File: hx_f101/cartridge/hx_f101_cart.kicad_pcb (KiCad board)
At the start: 2 copper layers, 100 x 85 mm, 10 parts, among them J1 Conn_02x25_Odd_Even, J2 CONN_02x17, U1 27C128, U2 74LS245, U3 74LS133, U4 74LS32, U5 74LS04, U6 74LS07, U7 74LS07, U8 74LS00

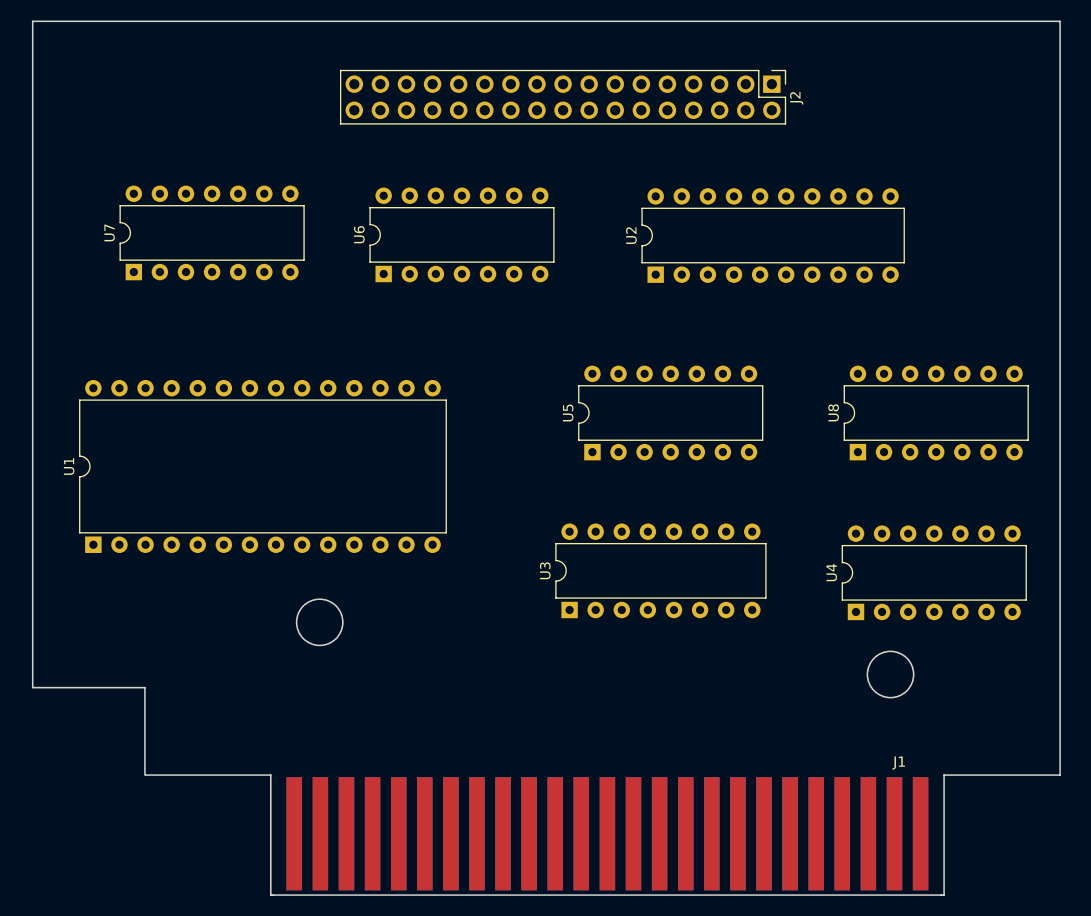
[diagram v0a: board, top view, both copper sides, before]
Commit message: Add files via upload
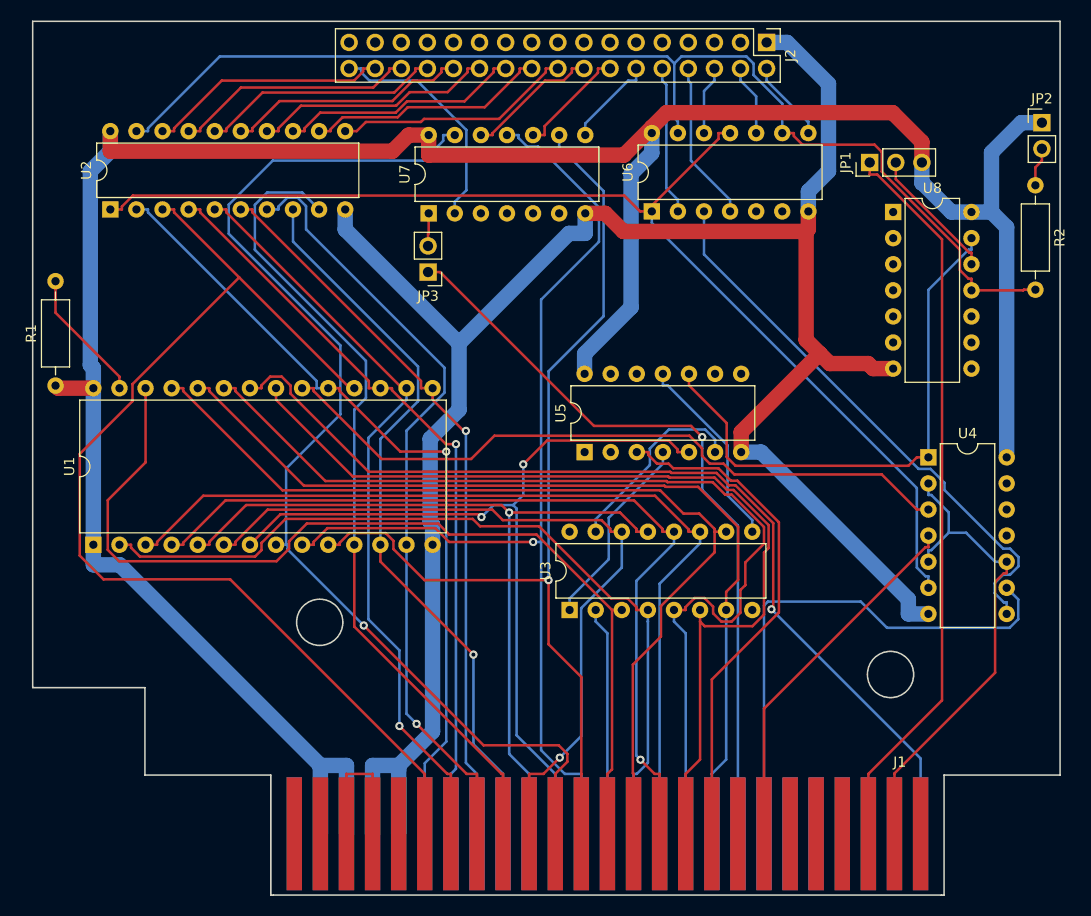
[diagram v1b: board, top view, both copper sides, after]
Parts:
- added JP1: Jumper_NC_Dual, Connector_PinHeader_2.54mm:PinHeader_1x03_P2.54mm_Vertical, F.Cu at (200.5, 70.7)
- added JP2: Jumper, Connector_PinHeader_2.54mm:PinHeader_1x02_P2.54mm_Vertical, F.Cu at (217.2, 66.9)
- added JP3: Jumper, Connector_PinHeader_2.54mm:PinHeader_1x02_P2.54mm_Vertical, F.Cu at (157.5, 81.4)
- added R1: 10K, Resistor_THT:R_Axial_DIN0207_L6.3mm_D2.5mm_P10.16mm_Horizontal, F.Cu at (121.2, 92.5)
- added R2: 330R, Resistor_THT:R_Axial_DIN0207_L6.3mm_D2.5mm_P10.16mm_Horizontal, F.Cu at (216.6, 73.0)
- moved U2 53.5 mm to (126.6, 75.3)
- moved U7 29.3 mm to (157.5, 75.7)
- moved U6 26.8 mm to (179.3, 75.5)
- moved U8 23.6 mm to (202.8, 75.6), turned to 0 degrees
- moved U4 16.6 mm to (206.2, 99.4), turned to 0 degrees
- moved J2 4.10 mm to (190.4, 59.1)
- moved U5 0.76 mm to (172.7, 98.9)
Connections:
- net P18 renamed PB18
- net P20 renamed PB20
- net P22 renamed PB22
- net P24 renamed PB24
- net P26 renamed PB26
- net P28 renamed PB28
- net P30 renamed PB30
- net P32 renamed PB32
- J1 pad 13: (no net) -> _WR
- J1 pad 14: (no net) -> _RD
- J1 pad 15: (no net) -> _RESET
- J1 pad 18: (no net) -> A15
- J1 pad 25: (no net) -> A14
- J1 pad 6: (no net) -> _RFSH
- J2 pad 1: (no net) -> GND
- J2 pad 10: (no net) -> PB10
- J2 pad 12: (no net) -> PB12
- J2 pad 14: (no net) -> PB14
- J2 pad 16: (no net) -> PB16
- J2 pad 2: (no net) -> PB2
- J2 pad 34: (no net) -> PB34
- J2 pad 4: (no net) -> PB4
- J2 pad 6: (no net) -> PB6
- J2 pad 8: (no net) -> PB8
- U1 pad 20: _SLTSL -> _ROM_CE
- U1 pad 27: (no net) -> Net-(R1-Pad2)
- U2 pad 1: (no net) -> _RE
- U2 pad 19: Net-(U2-Pad19) -> _CS
- U3 pad 1: (no net) -> Net-(U3-Pad1)
- U3 pad 10: (no net) -> A8
- U3 pad 11: (no net) -> A7
- U3 pad 12: (no net) -> A6
- U3 pad 13: (no net) -> A5
- U3 pad 14: (no net) -> A4
- U3 pad 15: (no net) -> Net-(U3-Pad15)
- U3 pad 2: (no net) -> A14
- U3 pad 3: (no net) -> A13
- U3 pad 4: (no net) -> A12
- U3 pad 5: (no net) -> A11
- U3 pad 6: (no net) -> A10
- U3 pad 7: (no net) -> A9
- U3 pad 9: Net-(U2-Pad19) -> Net-(U3-Pad9)
- U4 pad 1: (no net) -> Net-(U4-Pad1)
- U4 pad 10: (no net) -> _SLTSL
- U4 pad 13: Net-(U2-Pad19) -> (no net)
- U4 pad 2: (no net) -> _SLTSL
- U4 pad 3: (no net) -> _ROM_CE
- U4 pad 4: (no net) -> _RD
- U4 pad 5: (no net) -> _SLTSL
- U4 pad 6: (no net) -> _RE
- U4 pad 8: Net-(U4-Pad8) -> _WE
- U4 pad 9: (no net) -> _WR
- U5 pad 10: Net-(U5-Pad10) -> Net-(U4-Pad1)
- U5 pad 11: (no net) -> Net-(U3-Pad9)
- U5 pad 3: (no net) -> A15
- U5 pad 4: (no net) -> Net-(U3-Pad1)
- U5 pad 5: (no net) -> A3
- U5 pad 6: (no net) -> Net-(U3-Pad15)
- U6 pad 1: (no net) -> _RE
- U6 pad 10: (no net) -> PB4
- U6 pad 11: (no net) -> _RE
- U6 pad 12: (no net) -> PB6
- U6 pad 13: (no net) -> _CS
- U6 pad 2: (no net) -> PB10
- U6 pad 3: (no net) -> _WE
- U6 pad 4: (no net) -> PB8
- U6 pad 8: (no net) -> PB2
- U6 pad 9: (no net) -> _CS
- U7 pad 1: (no net) -> Net-(JP3-Pad2)
- U7 pad 10: (no net) -> PB14
- U7 pad 11: (no net) -> A1
- U7 pad 12: (no net) -> PB16
- U7 pad 13: (no net) -> A2
- U7 pad 2: (no net) -> PB34
- U7 pad 8: (no net) -> PB12
- U7 pad 9: (no net) -> A0
- U8 pad 1: Net-(U4-Pad8) -> (no net)
- U8 pad 11: (no net) -> _CS
- U8 pad 12: (no net) -> Net-(JP1-Pad2)
- U8 pad 13: (no net) -> Net-(U4-Pad1)
- U8 pad 9: Net-(U5-Pad10) -> (no net)
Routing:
- net 5V: track 0.00 -> 254.4 mm
- net GND: track 0.00 -> 199.6 mm
- net _RE: track 0.00 -> 113.7 mm
- net _CS: track 0.00 -> 113.1 mm
- net A2: track 0.00 -> 110.2 mm, vias 0 -> 1
- net D6: track 0.00 -> 107.8 mm
- net A1: track 0.00 -> 102.6 mm, vias 0 -> 1
- net A11: track 0.00 -> 98.7 mm
- net A0: track 0.00 -> 97.7 mm, vias 0 -> 1
- net A13: track 0.00 -> 95.1 mm
- net _CS1: track 0.00 -> 94.3 mm, vias 0 -> 1
- net A8: track 0.00 -> 92.8 mm
- net A10: track 0.00 -> 92.3 mm
- net A9: track 0.00 -> 89.3 mm
- net A7: track 0.00 -> 88.7 mm
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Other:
- outline, holes or cut-outs redrawn
- net class Power added: clearance 0.4, trace_width 1.5, via_dia 2, via_drill 1
